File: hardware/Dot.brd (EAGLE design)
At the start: 25.4 x 31.5 mm, 36 parts, among them IC1 CAT24M010TS, IC2 SI1145, U1 ATMEGA328P-MU-QFN32, U2 TMP102, U3 ISL29125, U4 9DoF IMU, U5 BMP18

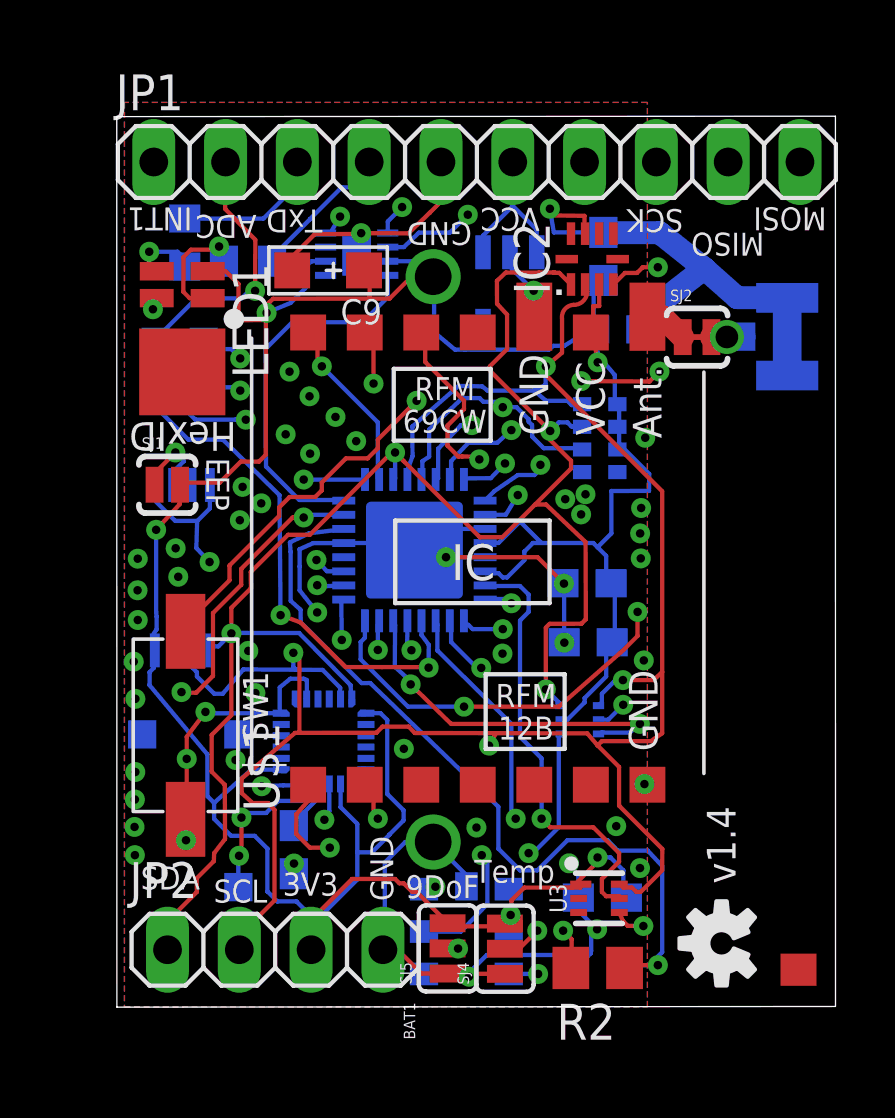
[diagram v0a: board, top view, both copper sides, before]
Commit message: Rearranging files
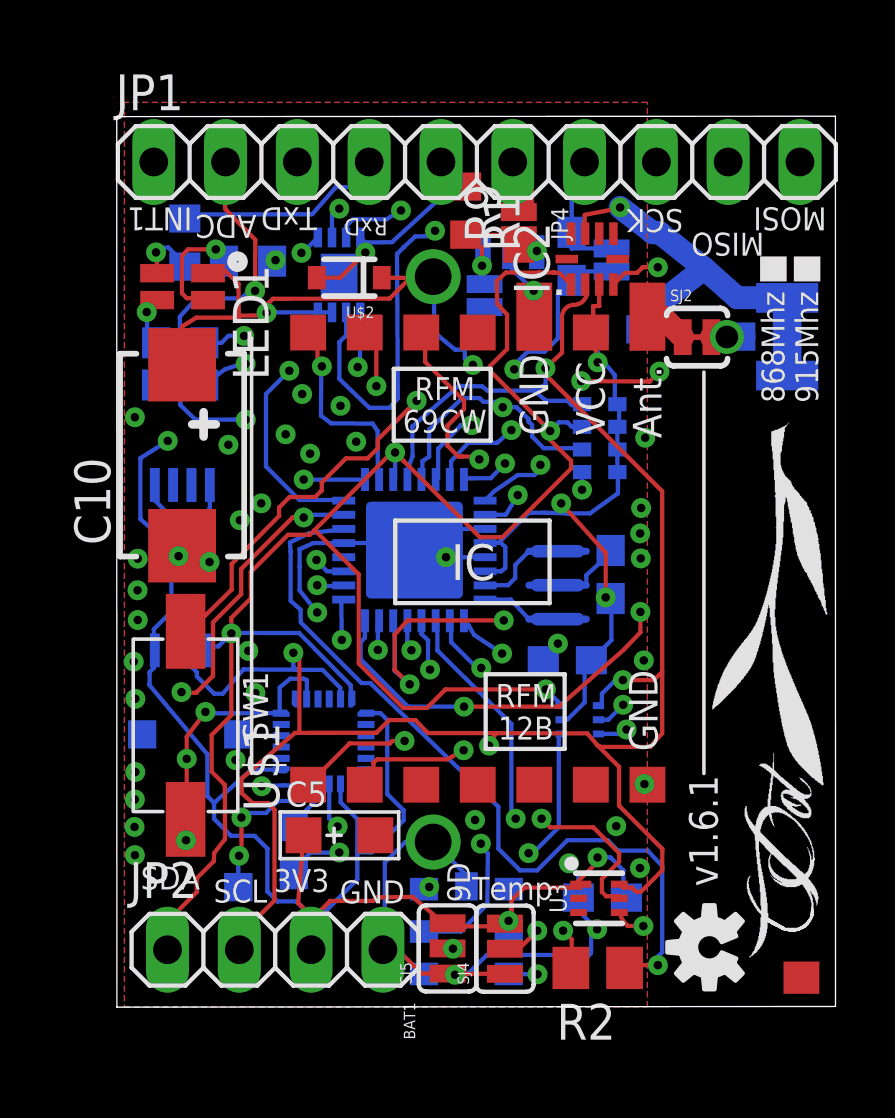
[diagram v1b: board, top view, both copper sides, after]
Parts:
- removed C6: 1uF, resistor:C0603
- removed C9: 100uf, Seeed-OPL-Capacitor:AVX-A
- removed SJ1: SOLDERJUMPERNO, SparkFun:SJ_2S-NO
- added C10: 1500uF 4V, adafruit:CT7343
- added C5: 100uf, Seeed-OPL-Capacitor:AVX-A
- added C7: 1uF, resistor:C0603
- added JP3, JP4: JUMPER-SMT_2_NO_NO-SILK, SparkFun-Jumpers:SMT-JUMPER_2_NO_NO-SILK
- added R1, R9: (no value), resistor:R0603
- added SJ3: SOLDERJUMPERNC2, SparkFun:SJ_2S-NOTRACE
- added U$2: DIODE-ZENER-BZT52, SparkFun:SOD-323
- added Y1: (no value), SparkFun-Clocks:RESONATOR-SMD-3.2X1.3
- R5: value 130Ω -> 67Ω
- R6, R8: value 30Ω -> 67Ω
- U$3: value AT45DB641E -> AT25SF081; device AT45DB641E:UDFN-8 -> AT25SF081:DFN-2X3
- moved R8 1.57 mm to (2.60, 24.0), turned to 180 degrees
- moved R4 1.48 mm to (2.60, 22.5)
- moved C2 0.97 mm to (16.3, 12.8)
- moved U$3 0.96 mm to (8.22, 26.4), turned to 270 degrees
- moved C3 0.89 mm to (17.8, 15.8), turned to 90 degrees
- moved LOGO1 0.45 mm to (21.3, 2.63)
- moved LED1 0.07 mm to (2.68, 26.0)
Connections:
- removed net INT_RGB: U1.7, U3.5
- removed net INT_UV: IC2.4, U1.8
- removed net N$2: IC1.A1, SJ1.1
- removed net TEMP_ALERT: U1.14, U2.3
- new net INT_MULTIPLE: IC2.4, R7.1, U1.14, U2.3, U3.5
- new net N$5: C7.2, JP1.7, JP3.2
- new net N$6: U1.7, Y1.3
- new net N$8: U1.8, Y1.1
- new net VIN_PIN: JP1.6, JP4.1, R9.2
- net +3V3: now also C10.+, C5.+, R7.8, SJ3.2, U$2.1, U$3.7, U$3.8; no longer C6.1, C9.+, SJ1.2, U$3.6
- net FLASH_CS: now also U$3.1; no longer U$3.4
- net GND: now also C10.-, C5.-, R1.1, U$2.2, U$3.4, Y1.2; no longer C6.2, C9.-, U$3.7, U$3.THERM
- net LED: now also R5.2; no longer R8.2
- net MISO: now also U$3.2; no longer U$3.8
- net MOSI: now also U$3.5; no longer U$3.1
- net RST: now also C7.1, JP3.1; no longer JP1.7
- net RXD: now also R6.2; no longer R5.2
- net SCK: now also U$3.6; no longer U$3.2
- net TXD: now also R8.2; no longer R6.2
- net VIN: now also JP4.2, R1.2, R9.1, SJ3.1; no longer JP1.6
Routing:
- net INT_MULTIPLE: track 0.00 -> 48.9 mm, vias 0 -> 6
- net INT_UV: track 17.1 -> 0.00 mm, vias 2 -> 0
- net INT_RGB: track 15.7 -> 0.00 mm, vias 1 -> 0
- net +3V3: track 131.1 -> 144.0 mm, vias 7 -> 11
- net TEMP_ALERT: track 12.8 -> 0.00 mm, vias 2 -> 0
- net SCK: track 41.4 -> 49.9 mm
- net MOSI: track 49.7 -> 55.9 mm
- net TXD: track 22.0 -> 28.0 mm, vias 1 -> 3
- net LED: track 19.0 -> 24.5 mm
- net RSDO: track 16.3 -> 11.3 mm
- net N$5: track 0.00 -> 4.66 mm
- net N$1: track 6.27 -> 2.00 mm, vias 2 -> 1
- net SDA: track 80.1 -> 84.4 mm
- net RST: track 19.3 -> 16.4 mm, vias 1 -> 2
- net N$2: track 2.90 -> 0.00 mm, vias 1 -> 0
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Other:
- board text added: "12.2017"
- board text added: "868Mhz"
- board text added: "915Mhz"
- board text added: "9D"
- board text added: "Mihai Galos"
- board text added: "RxD"
- board text added: "v1.6.1"
- board text removed: "9DoF"
- board text removed: "EEP"
- board text removed: "VCC"
- board text removed: "v1.4"
